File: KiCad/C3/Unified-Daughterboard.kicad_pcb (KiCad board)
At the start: 2 copper layers, 18 x 16.5 mm, 14 parts, among them J1 TYPE-C-31-M12_13, J2 SM04B-SRSS-TB(LF)(SN), U1 TPD4E05U06DQAR

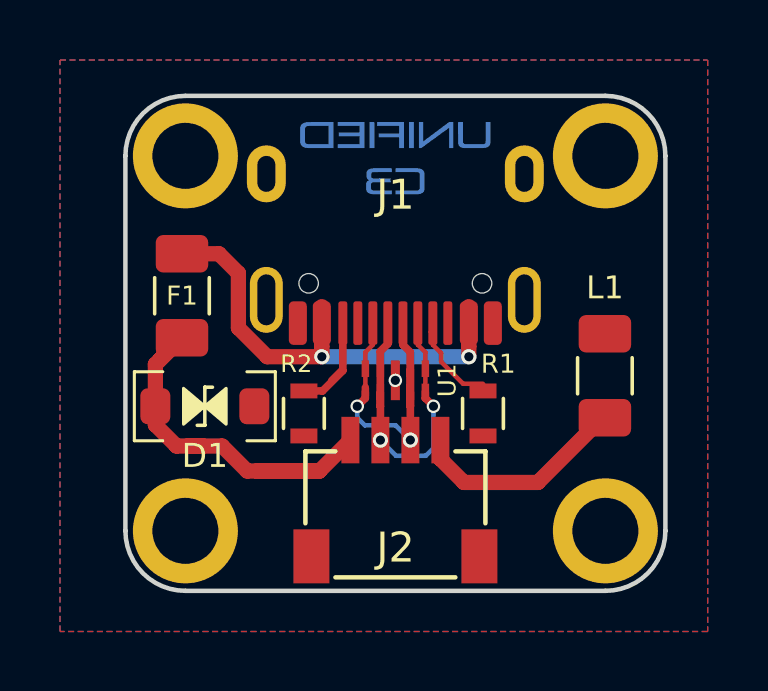
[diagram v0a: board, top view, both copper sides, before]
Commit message: repull
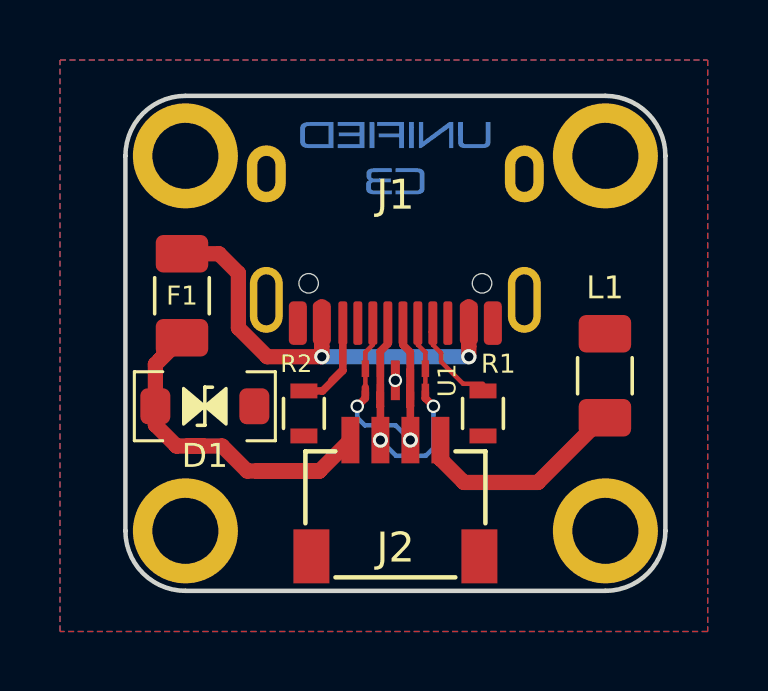
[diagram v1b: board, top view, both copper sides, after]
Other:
- net class Default removed
- net class Power removed
